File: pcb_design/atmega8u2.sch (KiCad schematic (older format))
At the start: 6 parts, among them U3 ATmega8U2-AU

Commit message: Add ISP header and bit more of USB thingo
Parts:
- added R? (x2): 1k, symbol Device:R
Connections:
- net labels added: PRGM_RST, PRGM_RX, PRGM_TX
- wire segments 19 -> 30
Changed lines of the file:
@@
 Wire Wire Line
 	4750 2450 4900 2450
+Text HLabel 6950 3800 2    50   Input ~ 0
+PRGM_RX
+Text HLabel 6950 3700 2    50   Input ~ 0
+PRGM_TX
+$Comp
+L Device:R R?
+U 1 1 6070CBFF
+P 6700 3600
+F 0 "R?" V 6493 3600 50  0000 C CNN
+F 1 "1k" V 6584 3600 50  0000 C CNN
+F 2 "" V 6630 3600 50  0001 C CNN
+F 3 "~" H 6700 3600 50  0001 C CNN
+	1    6700 3600
+	0    1    1    0
+$EndComp
+$Comp
+L Device:R R?
+U 1 1 6070D21B
+P 6700 3900
+F 0 "R?" V 6493 3900 50  0000 C CNN
+F 1 "1k" V 6584 3900 50  0000 C CNN
+F 2 "" V 6630 3900 50  0001 C CNN
+F 3 "~" H 6700 3900 50  0001 C CNN
+	1    6700 3900
+	0    1    1    0
+$EndComp
+Wire Wire Line
+	6300 3700 6550 3700
+Wire Wire Line
+	6550 3600 6550 3700
+Wire Wire Line
+	6300 3800 6550 3800
+Wire Wire Line
+	6550 3800 6550 3900
+Wire Wire Line
+	6850 3900 6900 3900
+Wire Wire Line
+	6900 3900 6900 3800
+Wire Wire Line
+	6900 3800 6950 3800
+Wire Wire Line
+	6850 3600 6900 3600
+Wire Wire Line
+	6900 3600 6900 3700
+Wire Wire Line
+	6900 3700 6950 3700
+Wire Wire Line
+	6300 4200 6500 4200
+Text HLabel 6500 4200 2    50   Input ~ 0
+PRGM_RST
 $EndSCHEMATC

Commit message: Move around
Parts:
- C6, C7: symbol Device:C_Small -> pcb_design-rescue:C_Small-Device
- Clk2: symbol Device:Crystal -> pcb_design-rescue:Crystal-Device
- R5, R6, R? (x2): symbol Device:R -> pcb_design-rescue:R-Device
- U3: symbol MCU_Microchip_ATmega:ATmega8U2-AU -> pcb_design-rescue:ATmega8U2-AU-MCU_Microchip_ATmega
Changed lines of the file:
@@
 	3750 2300 3900 2300
 $Comp
-L power:GND #PWR?
+L pcb_design-rescue:GND-power #PWR?
 U 1 1 6072964F
 P 3750 2300
@@
 $EndComp
 $Comp
-L Device:C_Small C?
+L pcb_design-rescue:C_Small-Device C?
 U 1 1 60729655
 P 4000 2450
@@
 $EndComp
 $Comp
-L Device:C_Small C?
+L pcb_design-rescue:C_Small-Device C?
 U 1 1 6072965B
 P 4000 2150
@@
 	3550 2600 3550 2450
 $Comp
-L Device:R R?
+L pcb_design-rescue:R-Device R?
 U 1 1 60729663
 P 3550 2300
@@
 	3900 2150 3900 2300
 $Comp
-L MCU_Microchip_ATmega:ATmega8U2-AU U?
+L pcb_design-rescue:ATmega8U2-AU-MCU_Microchip_ATmega U?
 U 1 1 6072966C
 P 5600 3100
@@
 $EndComp
 $Comp
-L Device:Crystal Clk?
+L pcb_design-rescue:Crystal-Device Clk?
 U 1 1 60729672
 P 4250 2300
@@
 	4250 2000 3550 2000
 $Comp
-L Device:R R?
+L pcb_design-rescue:R-Device R?
 U 1 1 60729681
 P 4600 2450
@@
 Connection ~ 5600 1600
 $Comp
-L power:GND #PWR?
+L pcb_design-rescue:GND-power #PWR?
 U 1 1 6072968C
 P 5600 4500
@@
 	5600 1600 5700 1600
 $Comp
-L power:+5V #PWR?
+L pcb_design-rescue:+5V-power #PWR?
 U 1 1 60729693
 P 5600 1600
@@
 PRGM_TX
 $Comp
-L Device:R R?
+L pcb_design-rescue:R-Device R?
 U 1 1 6070CBFF
 P 6700 3600
@@
 $EndComp
 $Comp
-L Device:R R?
+L pcb_design-rescue:R-Device R?
 U 1 1 6070D21B
 P 6700 3900

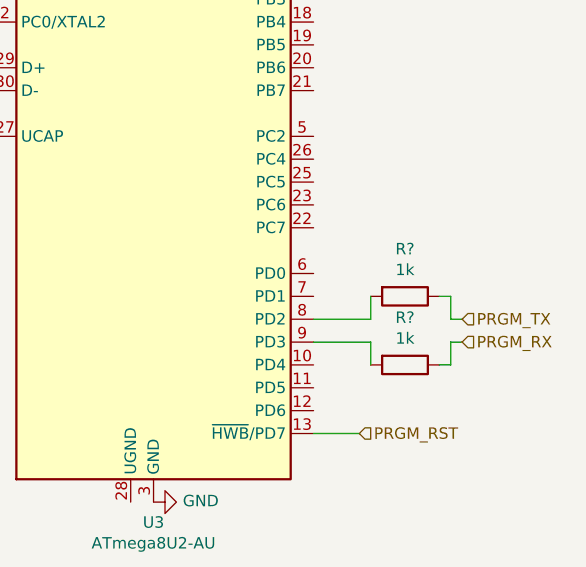
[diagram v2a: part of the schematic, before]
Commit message: Make PCB design
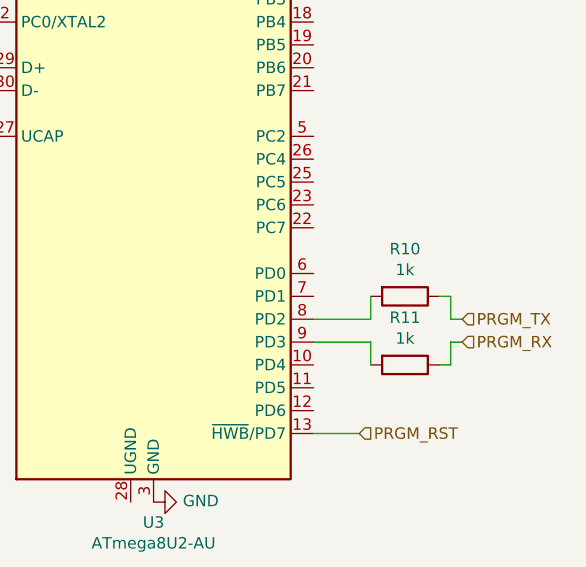
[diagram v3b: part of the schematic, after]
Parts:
- R10, R11: renamed from R?; footprint (none) -> Resistor_SMD:R_0201_0603Metric
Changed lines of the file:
@@
 PRGM_TX
 $Comp
-L pcb_design-rescue:R-Device R?
+L pcb_design-rescue:R-Device R10
 U 1 1 6070CBFF
 P 6700 3600
-F 0 "R?" V 6493 3600 50  0000 C CNN
+F 0 "R10" V 6493 3600 50  0000 C CNN
 F 1 "1k" V 6584 3600 50  0000 C CNN
-F 2 "" V 6630 3600 50  0001 C CNN
+F 2 "Resistor_SMD:R_0201_0603Metric" V 6630 3600 50  0001 C CNN
 F 3 "~" H 6700 3600 50  0001 C CNN
 	1    6700 3600
@@
 $EndComp
 $Comp
-L pcb_design-rescue:R-Device R?
+L pcb_design-rescue:R-Device R11
 U 1 1 6070D21B
 P 6700 3900
-F 0 "R?" V 6493 3900 50  0000 C CNN
+F 0 "R11" V 6493 3900 50  0000 C CNN
 F 1 "1k" V 6584 3900 50  0000 C CNN
-F 2 "" V 6630 3900 50  0001 C CNN
+F 2 "Resistor_SMD:R_0201_0603Metric" V 6630 3900 50  0001 C CNN
 F 3 "~" H 6700 3900 50  0001 C CNN
 	1    6700 3900
